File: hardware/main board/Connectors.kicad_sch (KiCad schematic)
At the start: 26 parts, among them J1 USB4145-03-0070-C, J10 M80-5100622, J11 M80-5101422, J14 Conn_01x05, J16 TagConnect, J2 M80-5100442, J3 M80-5100442, J4 M300-MV10345M1, J5 M300-MV10345M1, J6 M80-5100442, J7 M80-5100622, J8 M80-5102022, J9 M300-MV30645M1, T1 HX1188NL

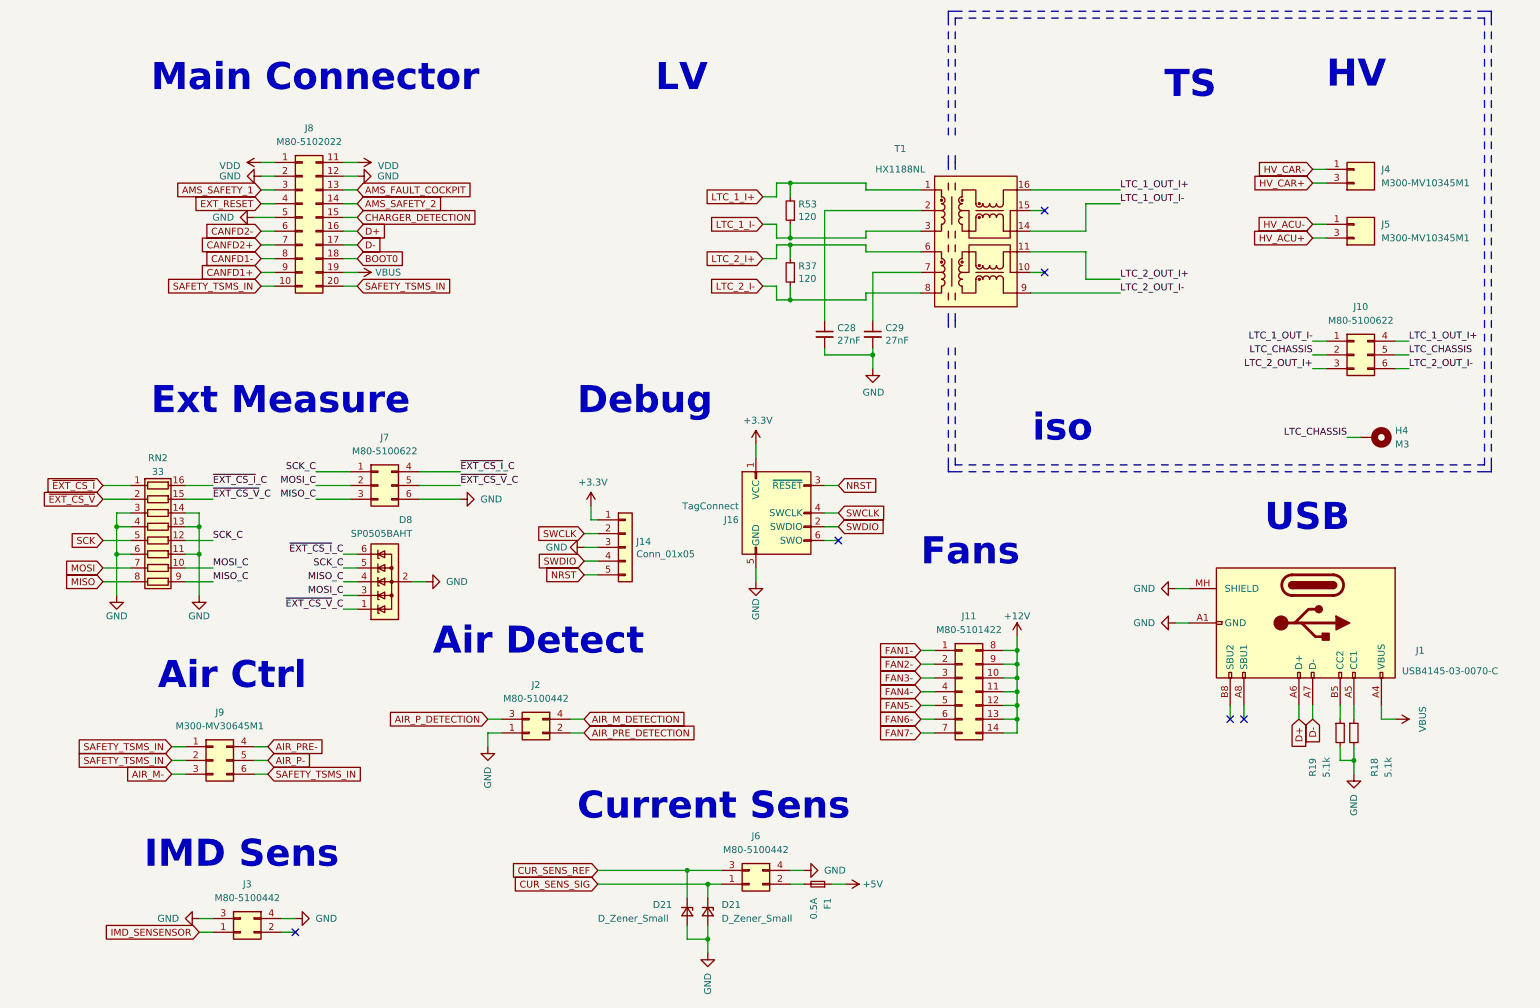
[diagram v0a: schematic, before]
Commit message: done power plane layout
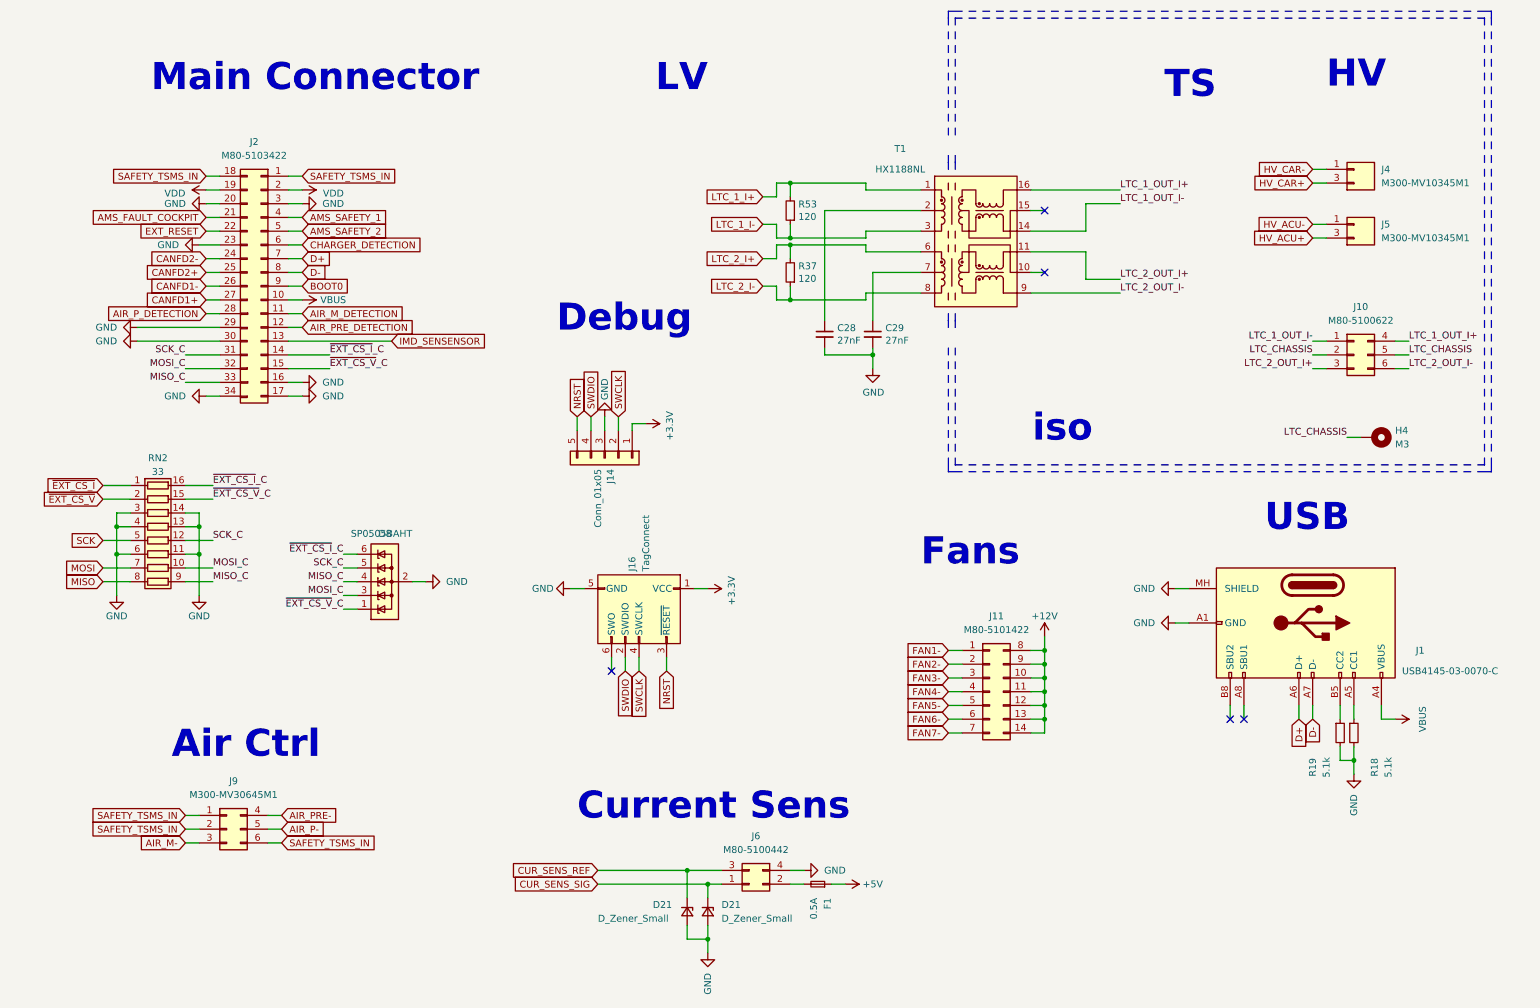
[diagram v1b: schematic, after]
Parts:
- removed J2, J3: M80-5100442, Samacsys:M80-51004YY, symbol Samacsys2:M80-5100442
- removed J7: M80-5100622, Samacsys:M80-51006YY, symbol Samacsys2:M80-5100622
- removed J8: M80-5102022, Samacsys:M80-51020YY, symbol Samacsys2:M80-5102022
- added J2: M80-5103422, Samacsys:M80-51034YY, symbol Samacsys2:M80-5103422
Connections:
- net AIR_M_DETECTION: now also J2.11
- net AIR_PRE_DETECTION: now also J2.12
- net AIR_P_DETECTION: now also J2.28
- net AMS_FAULT_COCKPIT: now also J2.21
- net AMS_SAFETY_1: now also J2.4
- net AMS_SAFETY_2: now also J2.5
- net BOOT0: now also J2.9
- net CANFD1+: now also J2.27
- net CANFD1-: now also J2.26
- net CANFD2+: now also J2.25
- net CANFD2-: now also J2.24
- net CHARGER_DETECTION: now also J2.6
- net D+: now also J2.7
- net D-: now also J2.8
- net EXT_RESET: now also J2.22
- net GND: now also J2.16, J2.17, J2.20, J2.23, J2.29, J2.3, J2.30, J2.34
- net IMD_SENSENSOR: now also J2.13
- net MISO_C: now also J2.33
- net MOSI_C: now also J2.32
- net SAFETY_TSMS_IN: now also J2.1, J2.18
- net SCK_C: now also J2.31
- net VBUS: now also J2.10
- net VDD: now also J2.19, J2.2
- net ~{EXT_CS_I}_C: now also J2.14
- net ~{EXT_CS_V}_C: now also J2.15
- no-connect marks 6 -> 5
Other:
- note removed: "Air Detect"
- note removed: "Ext Measure"
- note removed: "IMD Sens"
- moved on the sheet: J11, J14, J16, J9
